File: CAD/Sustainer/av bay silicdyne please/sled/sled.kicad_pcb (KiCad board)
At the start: 2 copper layers, 172.2 x 33.7 mm, 28 parts, among them J2 Conn_01x02, SW1 SW_DIP_x01, SW2 SW_DIP_x01, SW3 SW_DIP_x01, SW4 SW_DIP_x01, SW5 SW_SPDT

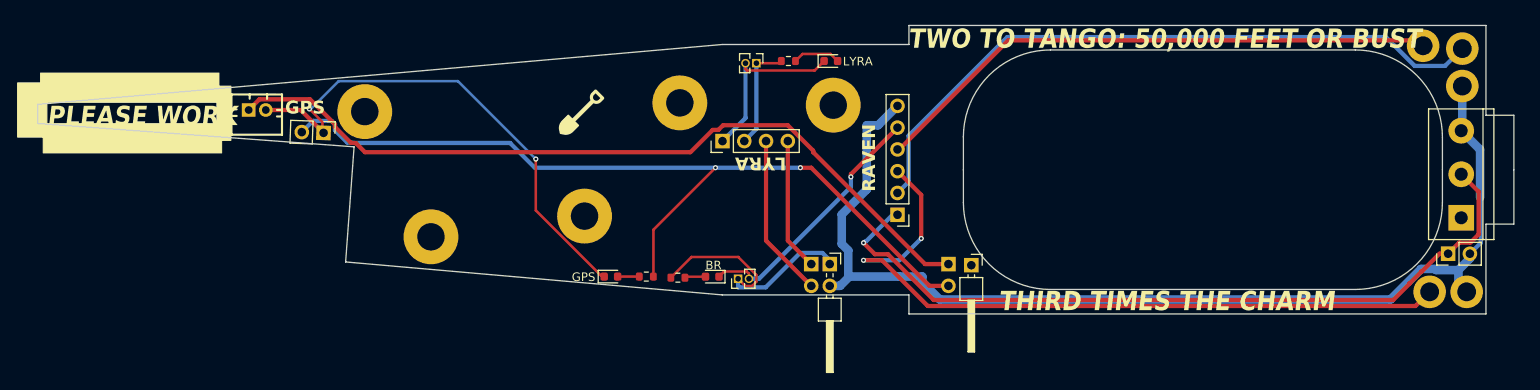
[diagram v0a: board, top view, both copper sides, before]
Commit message: work
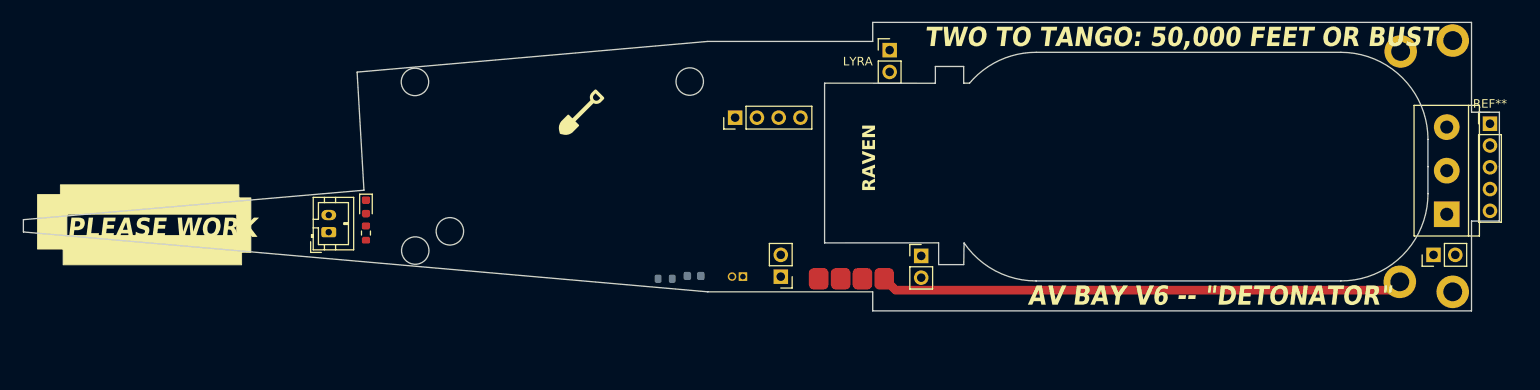
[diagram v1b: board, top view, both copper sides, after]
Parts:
- removed BR1: ~, Connector_PinHeader_2.54mm:PinHeader_1x06_P2.54mm_Vertical
- removed BT1: Battery, Connector_PinHeader_1.27mm:PinHeader_1x02_P1.27mm_Vertical
- removed D3: LED, LED_SMD:LED_0603_1608Metric
- removed GPS1: ~, Connector_PinHeader_2.54mm:PinHeader_1x02_P2.54mm_Vertical
- removed H10, H6: MountingHole_Pad, MountingHole:MountingHole_2.2mm_M2_DIN965_Pad
- removed R3: 1k, Resistor_SMD:R_0603_1608Metric
- removed SW3: SW_DIP_x01, Connector_PinHeader_2.54mm:PinHeader_2x01_P2.54mm_Horizontal
- removed SW4: SW_DIP_x01, Connector_PinHeader_2.54mm:PinHeader_1x01_P2.54mm_Horizontal
- added J1: Conn_01x02, Connector_PinHeader_2.54mm:PinHeader_1x02_P2.54mm_Vertical, F.Cu at (175.0, 46.0)
- added J3: Conn_01x04, .pretty:4 pads 2.54mm spacign, F.Cu at (166.8, 72.6)
- added REF**: PinHeader_1x05_P2.54mm_Vertical, Connector_PinHeader_2.54mm:PinHeader_1x05_P2.54mm_Vertical, F.Cu at (245.0, 54.6)
- BT2, D1, R1: moved to B.Cu
- BT3: footprint easyeda2kicad:CONN-TH_2P-P2.00_PH-2AK -> Connector_JST:JST_PH_B2B-PH-K_1x02_P2.00mm_Vertical
- H1, H2, H3, H5: footprint MountingHole:MountingHole_3.2mm_M3_Pad -> MountingHole:MountingHole_3.2mm_M3
- H4: footprint MountingHole:MountingHole_3.2mm_M3_Pad -> MountingHole:MountingHole_2.2mm_M2_DIN965_Pad
- SW1: footprint Connector_PinHeader_2.54mm:PinHeader_2x01_P2.54mm_Horizontal -> Connector_PinHeader_2.54mm:PinHeader_1x02_P2.54mm_Vertical
- SW2: footprint Connector_PinHeader_2.54mm:PinHeader_2x01_P2.54mm_Horizontal -> Connector_PinHeader_2.54mm:PinHeader_1x02_P2.54mm_Vertical; moved to F.Cu
- moved H4 103.3 mm to (240.7, 44.9)
- moved H1 48.9 mm to (119.6, 49.7)
- moved D2 41.2 mm to (113.9, 64.3), turned to -90 degrees
- moved R2 36.8 mm to (113.9, 67.3), turned to -90 degrees
- moved H5 35.2 mm to (151.7, 49.6)
- moved H2 30.7 mm to (123.7, 67.1)
- moved D1 29.7 mm to (152.2, 72.3), turned to 180 degrees
- moved R1 29.2 mm to (148.8, 72.6), turned to 0 degrees
- moved BT2 24.9 mm to (157.9, 72.4), turned to 90 degrees
- moved H3 17.2 mm to (119.7, 69.4)
- moved BT3 16.5 mm to (109.6, 67.2), turned to 90 degrees
- moved SW1 10.7 mm to (178.7, 70.0), turned to 0 degrees
- moved H11 8.25 mm to (234.6, 46.1), turned to 0 degrees
- moved H9 7.88 mm to (234.5, 73.0), turned to 0 degrees
- moved SW2 3.85 mm to (162.3, 72.4), turned to 180 degrees
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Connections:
- BT3 pad 2: Net-(BT3--) -> /FLUCTUS NEG
- D2 pad 1: /BR_NEG -> /FLUCTUS NEG
- H11 pad 1: /BR_POS -> /PYRO POS
- H4 pad 1: unconnected-(H4-Pad1) -> /APOGEE
- H9 pad 1: /BR_POS -> /PYRO POS
- J2 pad 2: /BR_POS -> /PYRO POS
- R2 pad 2: Net-(BT1-+) -> Net-(BT3-+)
- SW1 pad 1: Net-(BT1-+) -> Net-(BT3-+)
- SW1 pad 2: /BR_POS -> /FLUCTUS POS
- SW5 pad 3: /BR_POS -> /PYRO POS
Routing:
- net /BR_POS: track 128.7 -> 0.00 mm
- net Net-(GPS1-VIN): track 100.0 -> 0.00 mm, vias 2 -> 0
- net Net-(BT3-+): track 93.0 -> 0.00 mm
- net /HEI: track 90.9 -> 0.00 mm, vias 1 -> 0
- net /MAIN: track 85.7 -> 0.00 mm, vias 2 -> 0
- net /APO_BACKUP: track 78.8 -> 0.00 mm
- net /APOGEE: track 66.8 -> 0.00 mm
- net /PYRO POS: track 0.00 -> 61.1 mm
- net Net-(BT3--): track 60.0 -> 0.00 mm, vias 2 -> 0
- net /BR_NEG: track 30.2 -> 0.00 mm, vias 1 -> 0
- net Net-(BT1-+): track 29.5 -> 0.00 mm
- net Net-(BT2--): track 20.6 -> 0.00 mm
- net Net-(LYRA1-SW+): track 19.1 -> 0.00 mm
- net Net-(LYRA1-SW-): track 15.5 -> 0.00 mm
- net Net-(BT2-+): track 12.7 -> 0.00 mm
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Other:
- outline, holes or cut-outs redrawn
- board text added: "AV BAY V6 -- {dblquote}DETONATOR{dblquote}"
- board text removed: "BR"
- board text removed: "GPS"
- board text removed: "THIRD TIMES THE CHARM"
